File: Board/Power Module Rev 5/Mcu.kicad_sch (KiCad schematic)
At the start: 4 parts, among them J4 Conn_ARM_SWD_TagConnect_TC203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, J4 USB_C_Receptacle_USB2.0, U1 STM32G491CCUx, U6 MB85RS64

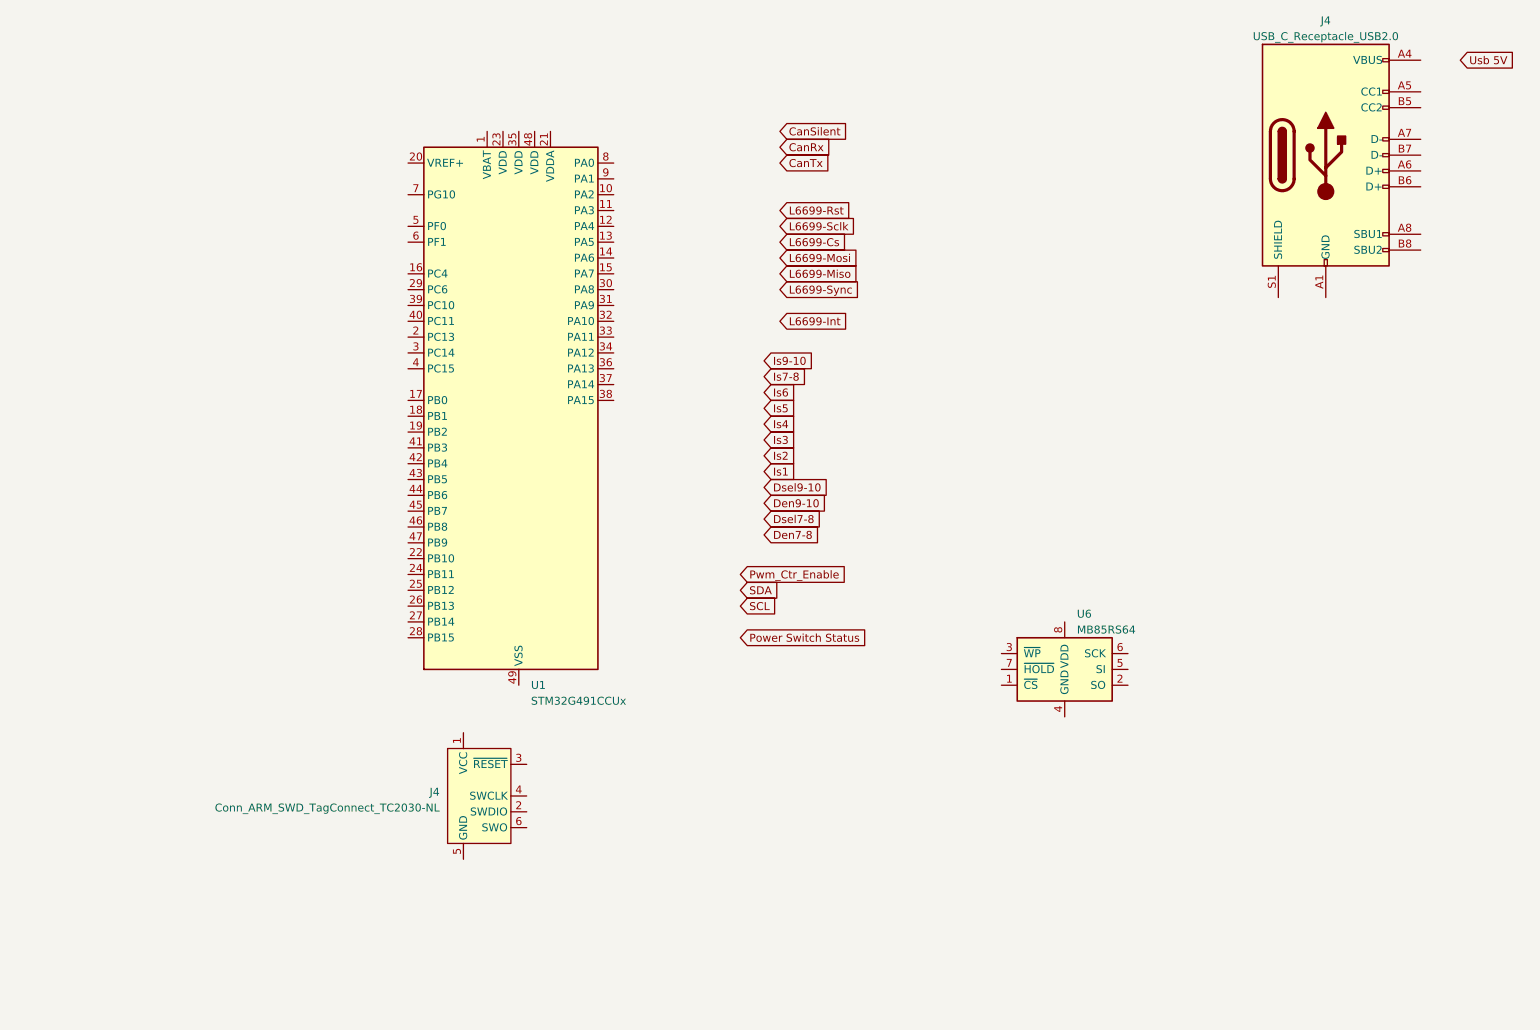
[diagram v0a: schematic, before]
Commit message: Update Board
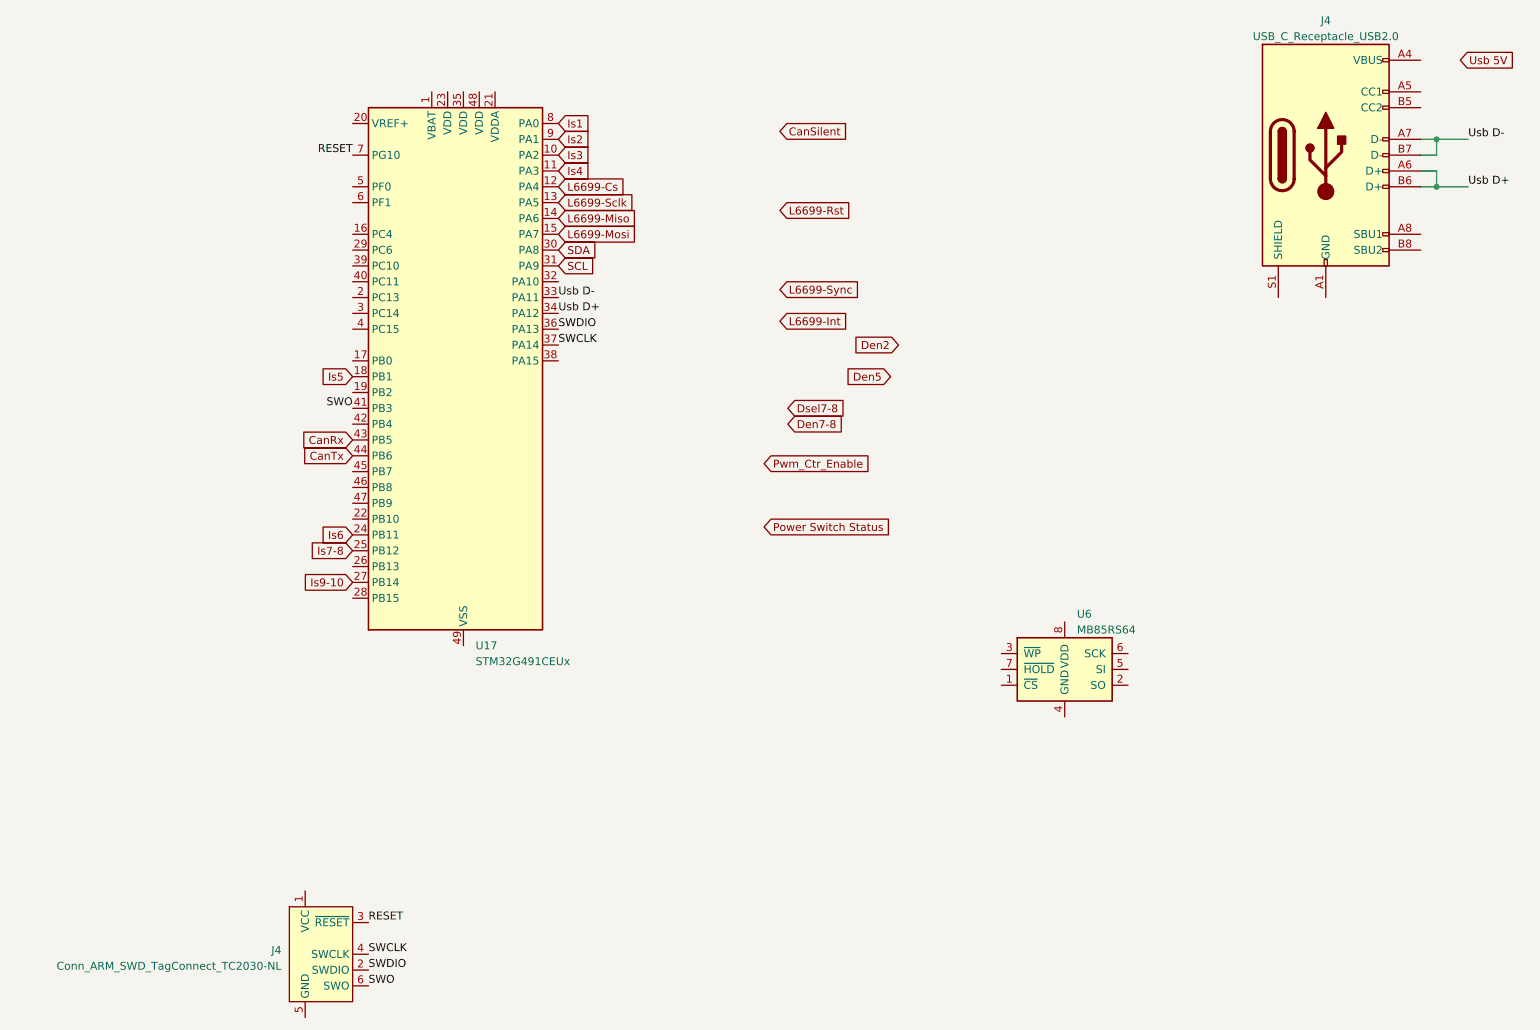
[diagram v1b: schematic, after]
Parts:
- removed U1: STM32G491CCUx, Package_DFN_QFN:QFN-48-1EP_7x7mm_P0.5mm_EP5.6x5.6mm, symbol MCU_ST_STM32G4:STM32G491CCUx
- added U17: STM32G491CEUx, Package_DFN_QFN:QFN-48-1EP_7x7mm_P0.5mm_EP5.6x5.6mm, symbol MCU_ST_STM32G4:STM32G491CEUx
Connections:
- net CanRx: now also U17.43 (PB5)
- net CanTx: now also U17.44 (PB6)
- net Is1: now also U17.8 (PA0)
- net Is2: now also U17.9 (PA1)
- net Is3: now also U17.10 (PA2)
- net Is4: now also U17.11 (PA3)
- net Is5: now also U17.18 (PB1)
- net Is6: now also U17.24 (PB11)
- net Is7-8: now also U17.25 (PB12)
- net Is9-10: now also U17.27 (PB14)
- net L6699-Cs: now also U17.12 (PA4)
- net L6699-Miso: now also U17.14 (PA6)
- net L6699-Mosi: now also U17.15 (PA7)
- net L6699-Sclk: now also U17.13 (PA5)
- net SCL: now also U17.31 (PA9)
- net SDA: now also U17.30 (PA8)
- net Usb D+: now reaches J4.A6 (D+)
- net Usb D+: now also J4.B6 (D+), U17.34 (PA12)
- net Usb D-: now reaches J4.A7 (D-)
- net Usb D-: now also J4.B7 (D-), U17.33 (PA11)
- net SWDIO: now reaches J4.2 (SWDIO)
- net SWDIO: now also U17.36 (PA13)
- net RESET: now reaches J4.3 (~{RESET})
- net RESET: now also U17.7 (PG10)
- net SWCLK: now reaches J4.4 (SWCLK)
- net SWCLK: now also U17.37 (PA14)
- net SWO: now reaches J4.6 (SWO)
- net SWO: now also U17.41 (PB3)
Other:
- moved on the sheet: J4
